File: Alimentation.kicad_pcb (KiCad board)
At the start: 2 copper layers, 50 x 50 mm, 21 parts, among them P1 Prise_Equilibrage, P10 CONN_01X02, P2 Prise_Alim, P3 Prise_Batterie, P4 ConnecteurBippeur, P5 CONN_01X04, P6 CAN_conn, P7 CAN_conn, P8 CONN_01X02, P9 CONN_01X02, U1 LD1084V

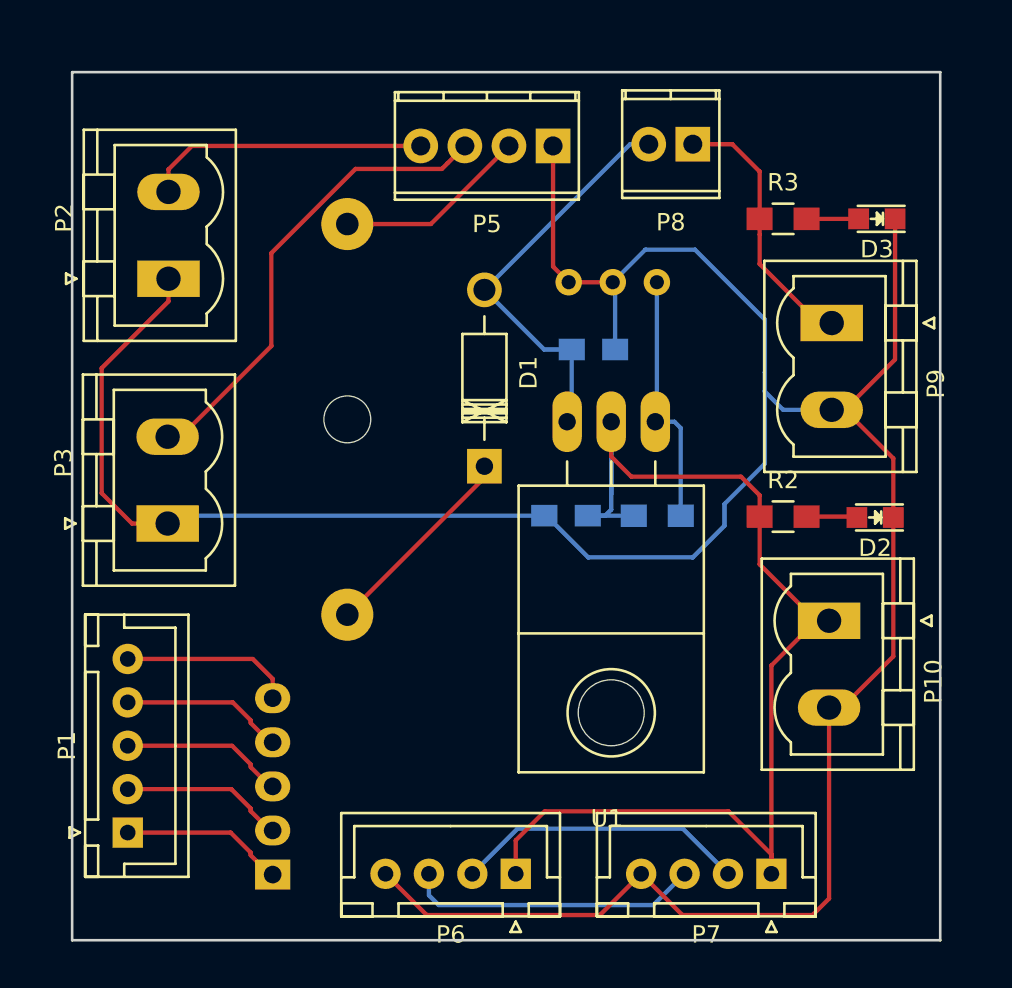
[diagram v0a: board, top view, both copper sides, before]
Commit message: routage terminé ?
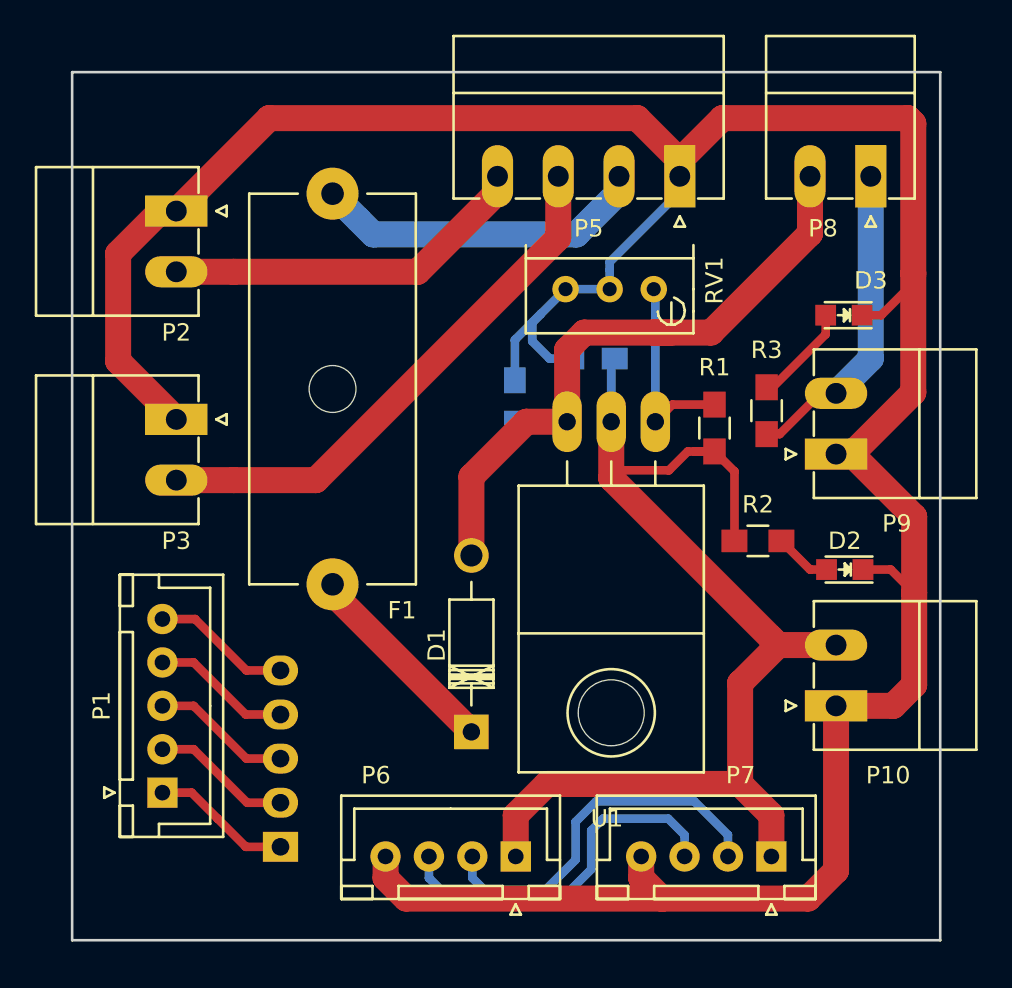
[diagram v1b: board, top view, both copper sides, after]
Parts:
- F1, R1, RV1: moved to F.Cu
- P10, P2, P3, P9: footprint Connectors_Phoenix:PhoenixContact_MSTBVA-G_02x5.00mm_Vertical -> Connectors_Phoenix:PhoenixContact_MC-G_02x3.50mm_Angled
- P5: footprint Terminal_Blocks:TerminalBlock_Pheonix_MPT-2.54mm_4pol -> Connectors_Phoenix:PhoenixContact_MC-G_04x3.50mm_Angled
- P8: footprint Terminal_Blocks:TerminalBlock_Pheonix_MPT-2.54mm_2pol -> Connectors_Phoenix:PhoenixContact_MC-G_02x3.50mm_Angled
- moved D1 15.3 mm to (123.0, 88.0)
- moved R3 11.1 mm to (140.0, 69.5), turned to 90 degrees
- moved P8 10.4 mm to (146.0, 56.0)
- moved C2 9.18 mm to (130.0, 66.5)
- moved P9 7.55 mm to (144.0, 72.0), turned to 90 degrees
- moved P5 7.51 mm to (135.0, 56.0)
- moved R1 6.03 mm to (137.0, 70.5), turned to 90 degrees
- moved P3 6.02 mm to (106.0, 70.0), turned to 270 degrees
- moved D3 5.87 mm to (144.5, 64.0)
- moved C1 5.44 mm to (125.5, 69.0), turned to 90 degrees
- moved P10 4.92 mm to (144.0, 86.5), turned to 90 degrees
- moved P2 3.93 mm to (106.0, 58.0), turned to 270 degrees
- moved D2 3.47 mm to (144.5, 78.7)
- moved P1 3.05 mm to (105.2, 91.5)
- moved R2 2.02 mm to (139.5, 77.0)
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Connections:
- P10 pad 1: +9V -> GND
- P10 pad 2: GND -> +9V
- P9 pad 1: Non_régulé -> GND
- P9 pad 2: GND -> Non_régulé
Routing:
- net Net-(C1-Pad1): track 23.7 -> 41.1 mm
- net Net-(F1-Pad2): track 11.2 -> 19.4 mm
- net Net-(P2-Pad2): track 16.4 -> 21.3 mm
- net CAN_H: track 16.9 -> 21.7 mm
- net CAN_L: track 16.9 -> 21.6 mm
- net Net-(P3-Pad2): track 27.2 -> 31.3 mm
- net GND: track 171.0 -> 174.4 mm
- net Non_régulé: track 15.4 -> 18.3 mm
- net Net-(D3-Pad2): track 3.00 -> 5.76 mm
- net +9V: track 69.5 -> 71.7 mm
- net Net-(R1-Pad2): track 14.7 -> 12.6 mm
- net Net-(P1-Pad5): track 9.94 -> 8.03 mm
- net Net-(P1-Pad2): track 9.43 -> 8.08 mm
- net Net-(P1-Pad4): track 9.39 -> 8.04 mm
- net Net-(P1-Pad3): track 9.41 -> 8.06 mm
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- added copper zone on B.Cu, net GND
- added copper zone on F.Cu, net GND
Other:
- net class DRC added: clearance 0.65, trace_width 0.5, via_dia 0.6, via_drill 0.4
- net class Interm added: clearance 0.4, trace_width 0.5, via_dia 0.6, via_drill 0.4
- net class PWR added: clearance 0.8, trace_width 1.5, via_dia 0.6, via_drill 0.4
